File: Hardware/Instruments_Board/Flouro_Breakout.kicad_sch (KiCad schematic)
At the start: 13 parts

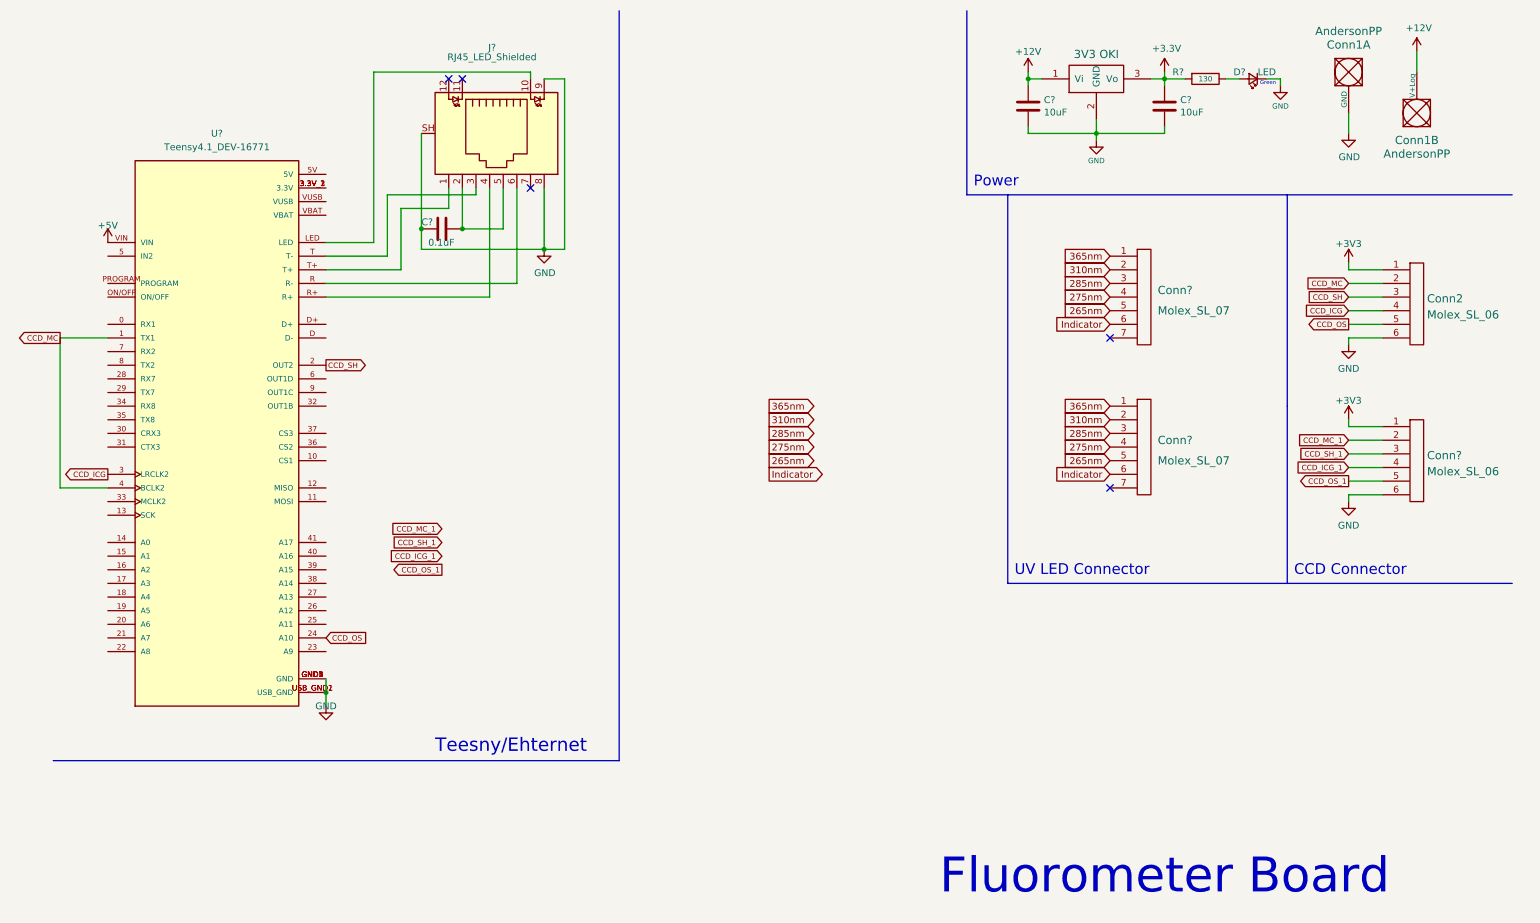
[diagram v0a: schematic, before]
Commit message: I Forgot
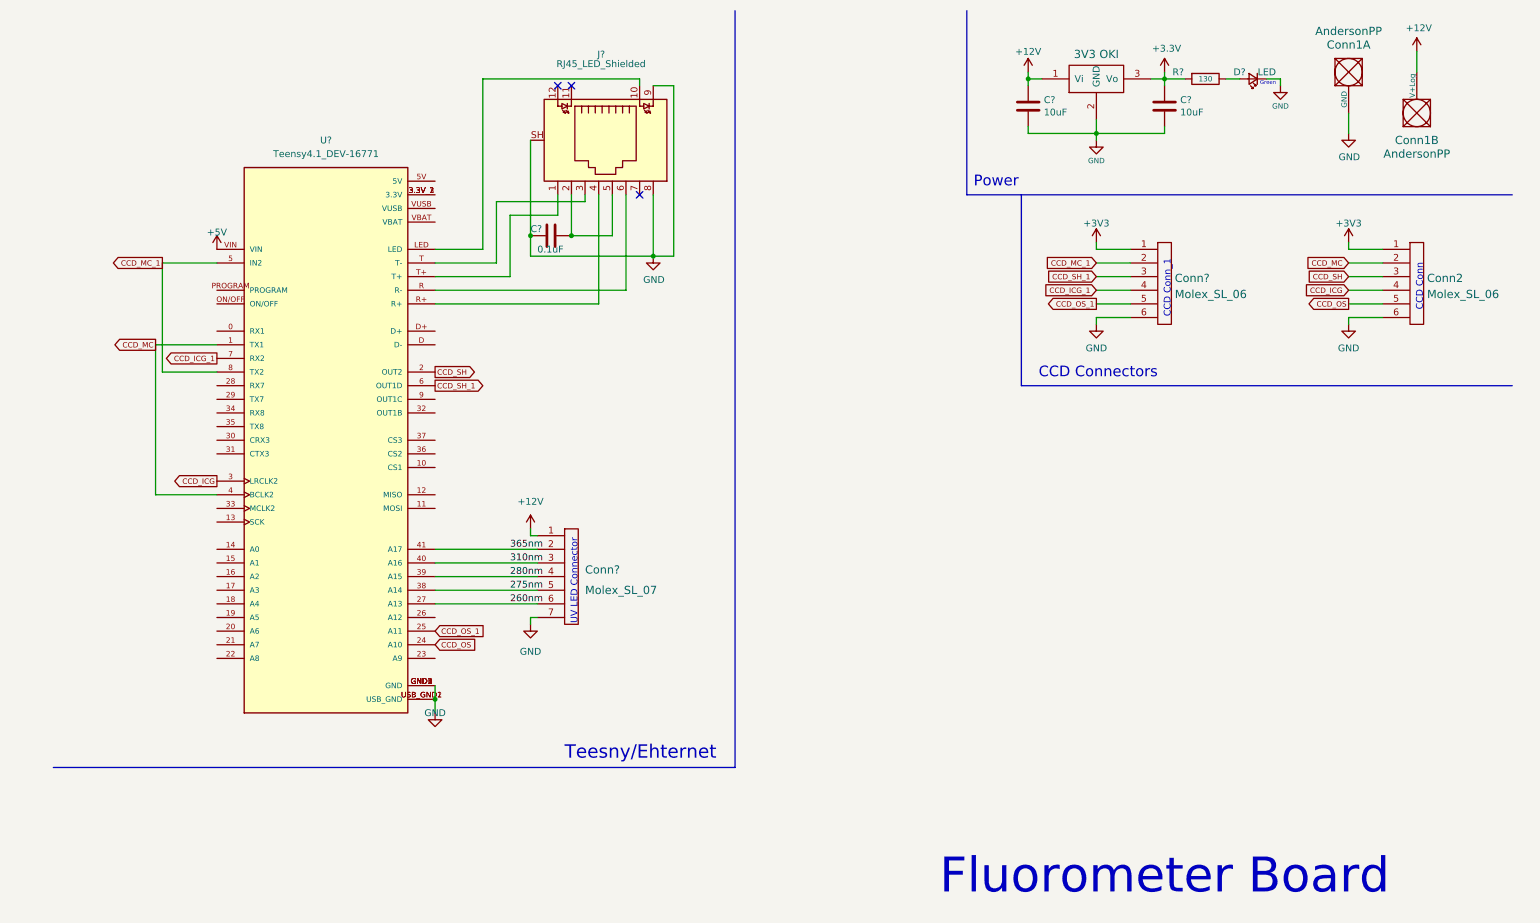
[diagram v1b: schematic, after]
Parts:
- removed Conn? (x2): Molex_SL_07, symbol MRDT_Connectors:Molex_SL_07
- added Conn?: Molex_SL_07, MRDT_Connectors:MOLEX_SL_07_Vertical, symbol MRDT_Connectors:Molex_SL_07
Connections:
- net  CCD_SH_1: now also U?.6 (OUT1D)
- net +12V: now also Conn?.1
- net 275nm: now also U?.38 (A14), Conn?.5
- net 310nm: now also U?.40 (A16), Conn?.3
- net 365nm: now also U?.41 (A17), Conn?.2
- net CCD_ICG_1: now also U?.7 (RX2)
- net CCD_MC_1: now also U?.5 (IN2), U?.8 (TX2)
- net CCD_OS_1: now also U?.25 (A11)
- net GND: now also Conn?.7
- net 260nm: now reaches U?.27 (A13)
- net 260nm: now also Conn?.6
- net 280nm: now reaches U?.39 (A15)
- net 280nm: now also Conn?.4
- no-connect marks 5 -> 3
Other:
- note added: "CCD Conn"
- note added: "CCD Conn_1"
- note added: "CCD Connectors"
- note removed: "CCD Connector"
- moved on the sheet: C?, Conn2, Conn?, J?, U?
